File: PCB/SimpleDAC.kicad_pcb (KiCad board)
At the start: 2 copper layers, 96.5 x 67 mm, 33 parts

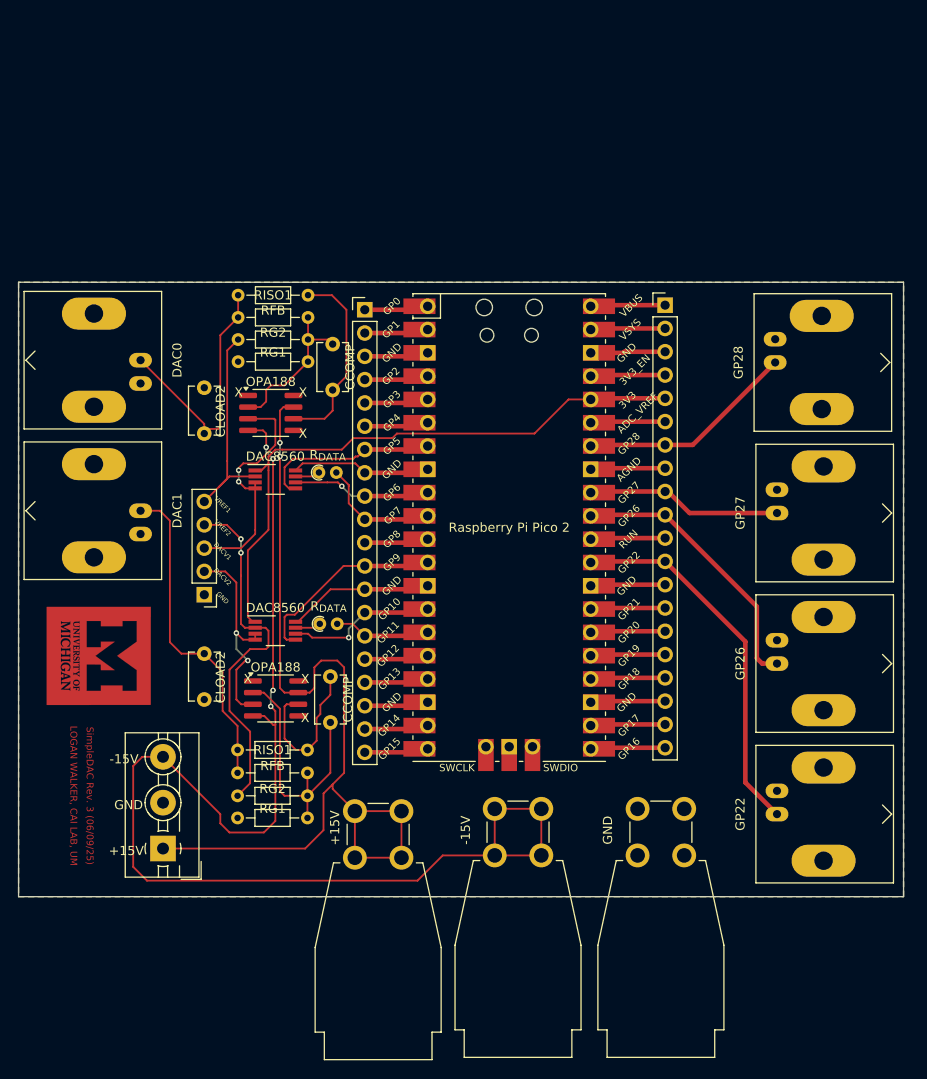
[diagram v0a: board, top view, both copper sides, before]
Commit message: Updating schematic
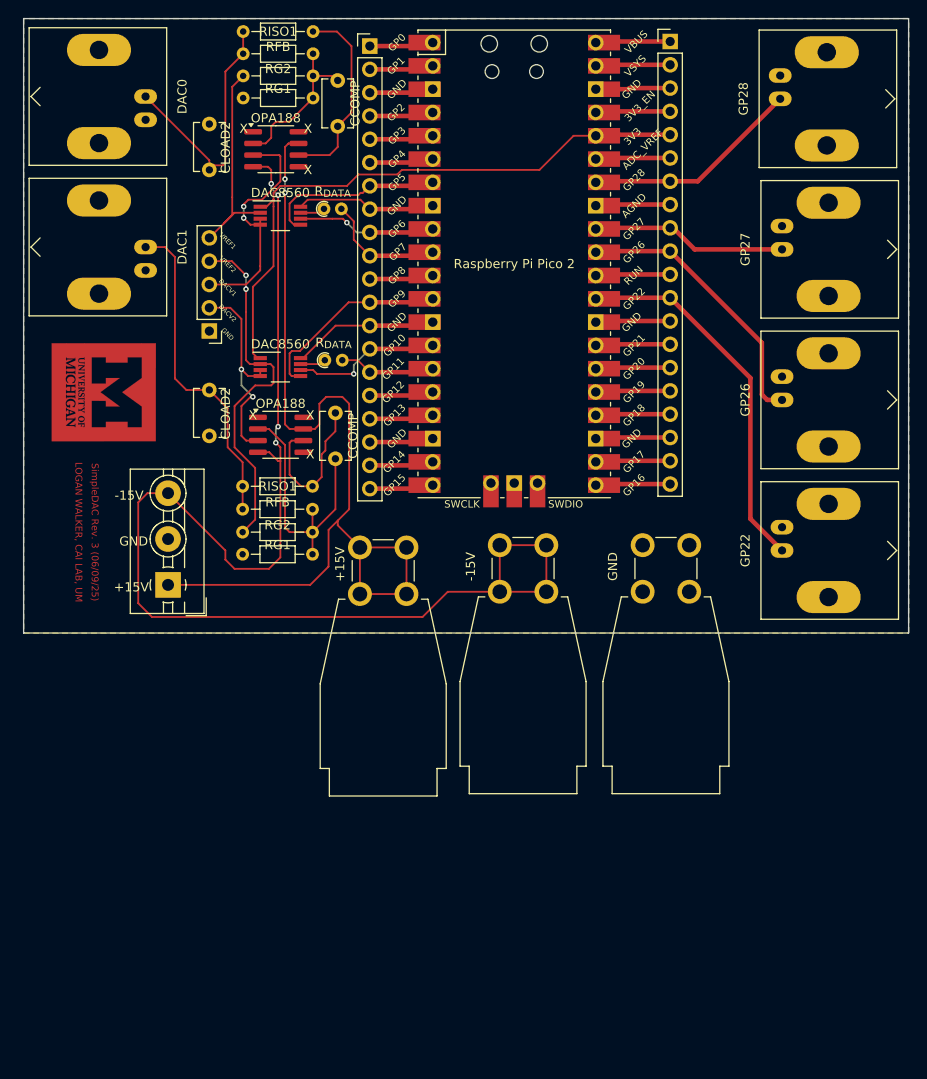
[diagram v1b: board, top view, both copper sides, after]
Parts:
- moved RG1 28.8 mm to (123.3, 103.9)
- moved   28.8 mm to (162.3, 48.0)
- moved   28.8 mm to (129.6, 48.5)
- moved   28.8 mm to (112.0, 79.6)
- moved +15V 28.8 mm to (128.5, 108.2)
- moved -15V 28.8 mm to (143.7, 108.0)
- moved CCOMP 28.8 mm to (126.0, 57.2)
- moved CCOMP 28.8 mm to (125.8, 93.5)
- moved CLOAD2 28.8 mm to (112.0, 91.0)
- moved CLOAD2 28.8 mm to (112.0, 62.0)
- moved DAC0 28.8 mm to (105.1, 54.0)
- moved DAC1 28.8 mm to (105.1, 70.4)
- moved DAC8560 28.8 mm to (119.8, 67.0)
- moved DAC8560 28.8 mm to (119.8, 83.5)
- moved G*** 28.8 mm to (100.5, 86.2)
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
